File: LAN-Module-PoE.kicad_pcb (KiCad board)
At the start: 2 copper layers, 28.6 x 53.3 mm, 91 parts, among them J1 HY931147C, J10 ProtoCastellatedHeader, J11 ProtoCastellatedHeader, J12 ProtoCastellatedHeader, J13 ProtoCastellatedHeader, J14 ProtoCastellatedHeader, J15 ProtoCastellatedHeader, J16 ProtoCastellatedHeader, J17 ProtoCastellatedHeader, J18 ProtoCastellatedHeader, J19 ProtoCastellatedHeader, J20 ProtoCastellatedHeader, J21 ProtoCastellatedHeader, J22 ProtoCastellatedHeader, J23 ProtoCastellatedHeader, J24 ProtoCastellatedHeader, J25 ProtoCastellatedHeader, J26 ProtoCastellatedHeader, J27 ProtoCastellatedHeader, J28 ProtoCastellatedHeader, J3 ProtoCastellatedHeader, J4 ProtoCastellatedHeader, J5 ProtoCastellatedHeader, J6 ProtoCastellatedHeader, J7 ProtoCastellatedHeader, J8 ProtoCastellatedHeader, J9 ProtoCastellatedHeader, SW1 RESET, U1 ESP32-U4WDH, U2 Si3404, U3 LV2842XLVDDCR, U4 RTL8201F, Y1 40MHz ±10ppm

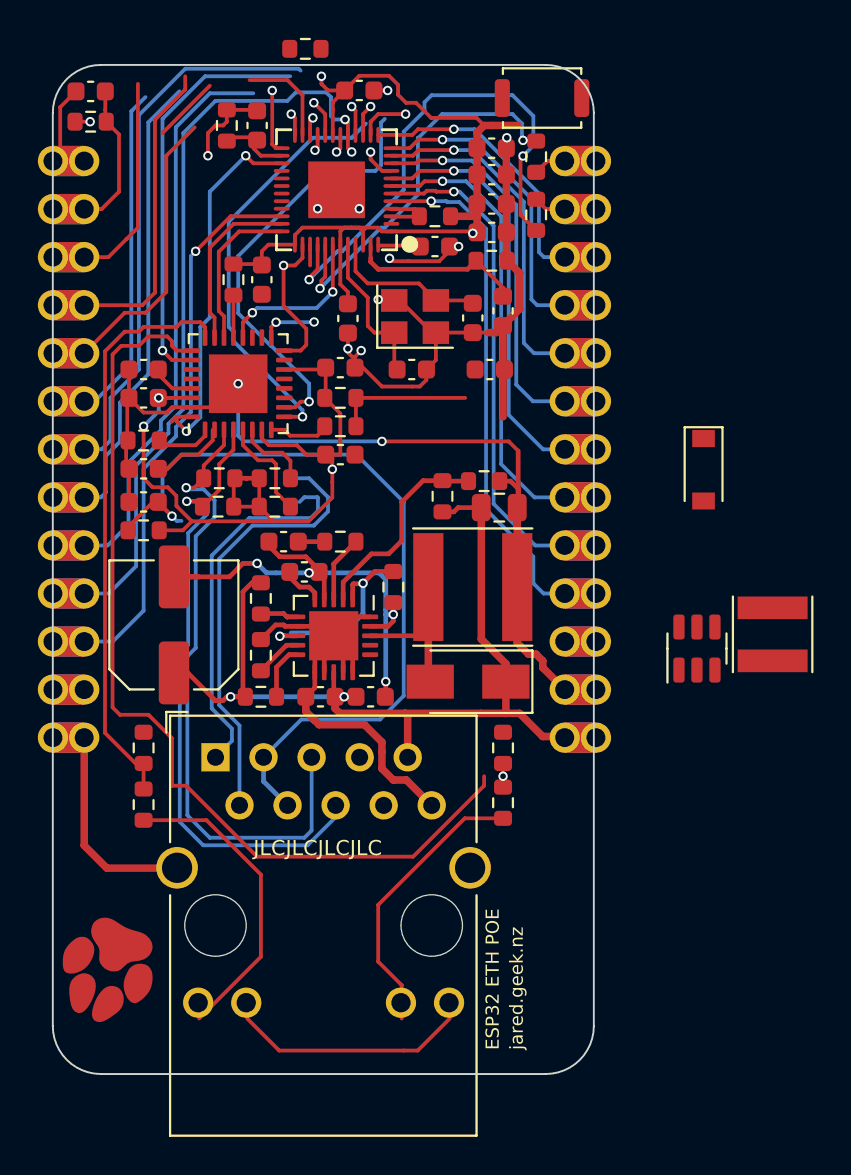
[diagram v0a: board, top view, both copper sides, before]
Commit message: Final revision of PoE variant
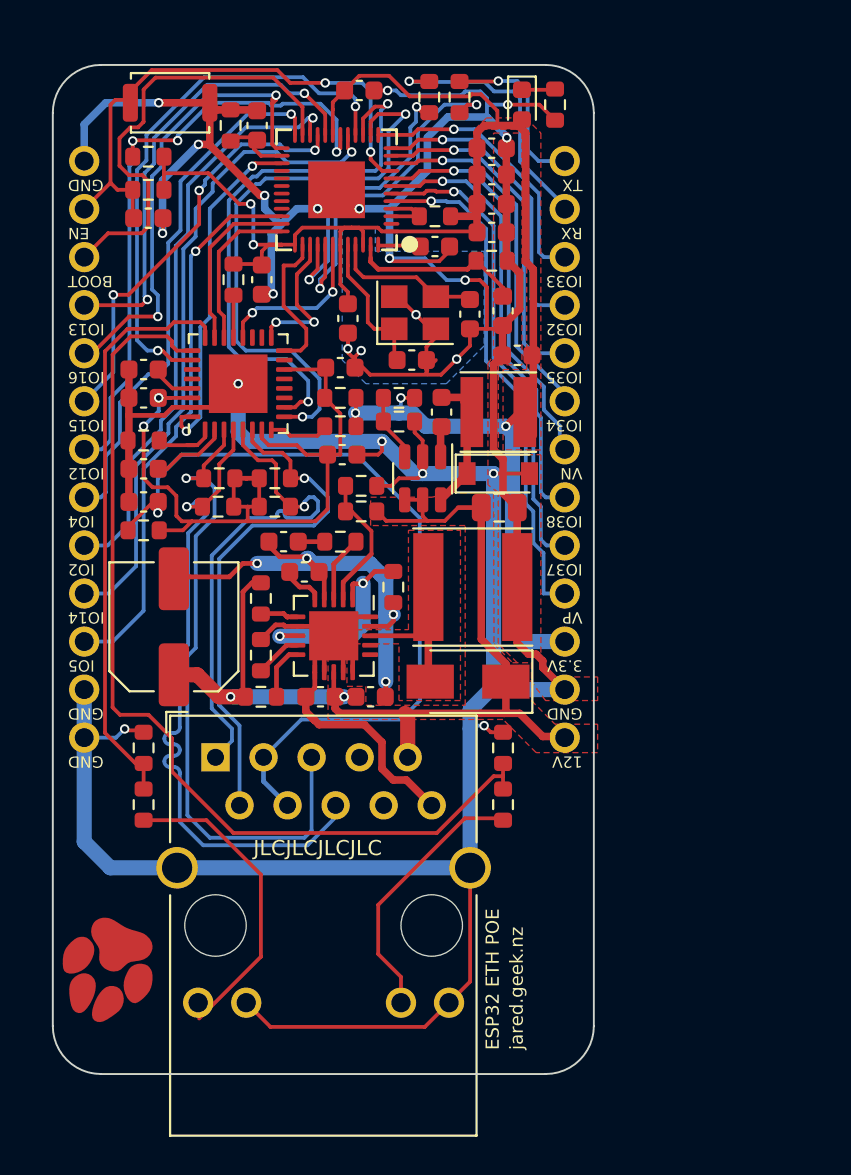
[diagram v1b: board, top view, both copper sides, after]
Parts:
- added C17: 100n, Capacitor_SMD:C_0603_1608Metric, F.Cu at (41.8, 43.8)
- added D3: Green, LED_SMD:LED_0603_1608Metric, F.Cu at (46.0, 27.5)
- added R26: 33k 1%, Resistor_SMD:R_0603_1608Metric, F.Cu at (39.5, 43.0)
- added R27: 10k 1%, Resistor_SMD:R_0603_1608Metric, F.Cu at (39.5, 44.2)
- added R28: 1k, Resistor_SMD:R_0603_1608Metric, F.Cu at (47.8, 27.5)
- J10, J11, J12, J13, J14, J15, J16, J17, J18, J19, J20, J21, J22, J23, J24, J25, J26, J27, J28, J3, J4, J5, J6, J7, J8, J9: footprint Visclib:ProtoCastellatedHeader_65mil -> Visclib:ProtoHeader_65mil
- L2: value 10uH -> 10uH 1A
- moved SW1 19.7 mm to (27.4, 27.4)
- moved L2 18.7 mm to (44.8, 43.8), turned to 0 degrees
- moved U3 17.1 mm to (40.8, 47.2), turned to -90 degrees
- moved D2 10.9 mm to (44.8, 47.0), turned to 0 degrees
- moved R5 10.1 mm to (26.2, 30.2), turned to 0 degrees
- moved R22 8.41 mm to (41.1, 27.1)
- moved C10 7.36 mm to (26.2, 33.5), turned to 180 degrees
- moved R24 6.50 mm to (37.5, 47.6)
- moved R4 5.13 mm to (42.7, 27.1), turned to -90 degrees
- moved R1 4.72 mm to (26.2, 32.0), turned to 0 degrees
- moved R23 4.37 mm to (37.5, 49.0), turned to 0 degrees
- moved C21 1.63 mm to (45.8, 40.8), turned to 180 degrees
- moved C12 0.50 mm to (40.2, 41.0)
- moved C13 0.25 mm to (43.2, 38.6)
- moved R2 0.20 mm to (30.6, 28.6)
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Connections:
- C1 pad 1: /VIN -> /12V
- C18 pad 1: /VIN -> /12V
- C27 pad 1: /VIN -> /12V
- C4 pad 1: /VIN -> /12V
- D1 pad 1: /VIN -> /12V
- D2 pad 1: unconnected-(D2-Pad1) -> Net-(C17-Pad2)
- D2 pad 2: unconnected-(D2-Pad2) -> GND
- J1 pad 9: /VIN -> /12V
- J1 pad SH: (no net) -> GND
- J15 pad 1: /3V3 -> +3V3
- J28 pad 1: /VIN -> /12V
- L2 pad 1: unconnected-(L2-Pad1) -> Net-(C17-Pad2)
- L2 pad 2: unconnected-(L2-Pad2) -> +3V3
- R19 pad 1: /VIN -> /12V
- R23 pad 2: /VIN -> /12V
- R6 pad 1: /VIN -> /12V
- U2 pad 13: /VIN -> /12V
- U3 pad 1: unconnected-(U3-Pad1) -> Net-(C17-Pad1)
- U3 pad 3: unconnected-(U3-Pad3) -> Net-(R26-Pad1)
- U3 pad 4: unconnected-(U3-Pad4) -> /12V
- U3 pad 5: unconnected-(U3-Pad5) -> /12V
- U3 pad 6: unconnected-(U3-Pad6) -> Net-(C17-Pad2)
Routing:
- net GND: track 116.9 -> 241.5 mm, vias 12 -> 22
- net /12V: track 0.00 -> 61.8 mm, vias 0 -> 2
- net /VIN: track 48.8 -> 0.00 mm, vias 2 -> 0
- net +3V3: track 51.6 -> 95.7 mm, vias 3 -> 5
- net /EN: track 9.56 -> 28.6 mm, vias 1 -> 2
- net /U0RXD: track 1.73 -> 14.0 mm, vias 0 -> 1
- net Net-(R22-Pad2): track 27.1 -> 15.0 mm
- net /BOOT: track 16.3 -> 23.9 mm
- net /POE_NEG: track 29.3 -> 21.8 mm
- net /U0TXD: track 1.76 -> 9.14 mm, vias 0 -> 1
- net Net-(C17-Pad2): track 0.00 -> 7.13 mm
- net /IO13: track 18.1 -> 24.2 mm, vias 1 -> 2
- net /ETH_RXD0: track 25.0 -> 30.9 mm
- net /IO16: track 18.4 -> 24.1 mm, vias 1 -> 2
- net /ETH_RXD1: track 24.4 -> 29.9 mm
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- added copper zone on F.Cu, net +3V3
- added copper zone on F.Cu, net /12V
- added copper zone on F.Cu, net /SWO
- added copper zone on B.Cu, net GND
- added copper zone on F.Cu, net GND
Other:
- board text added: "12V"
- board text added: "3.3V"
- board text added: "BOOT"
- board text added: "EN"
- board text added: "GND"
- board text added: "IO12"
- board text added: "IO13"
- board text added: "IO14"
- board text added: "IO15"
- board text added: "IO16"
- board text added: "IO2"
- board text added: "IO32"
- board text added: "IO33"
- board text added: "IO34"
- board text added: "IO35"
- board text added: "IO37"
- board text added: "IO38"
- board text added: "IO4"
- board text added: "IO5"
- board text added: "RX"
- board text added: "TX"
- board text added: "VN"
- board text added: "VP"
